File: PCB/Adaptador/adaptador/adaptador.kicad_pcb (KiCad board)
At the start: 2 copper layers, 38.1 x 41.9 mm, 4 parts

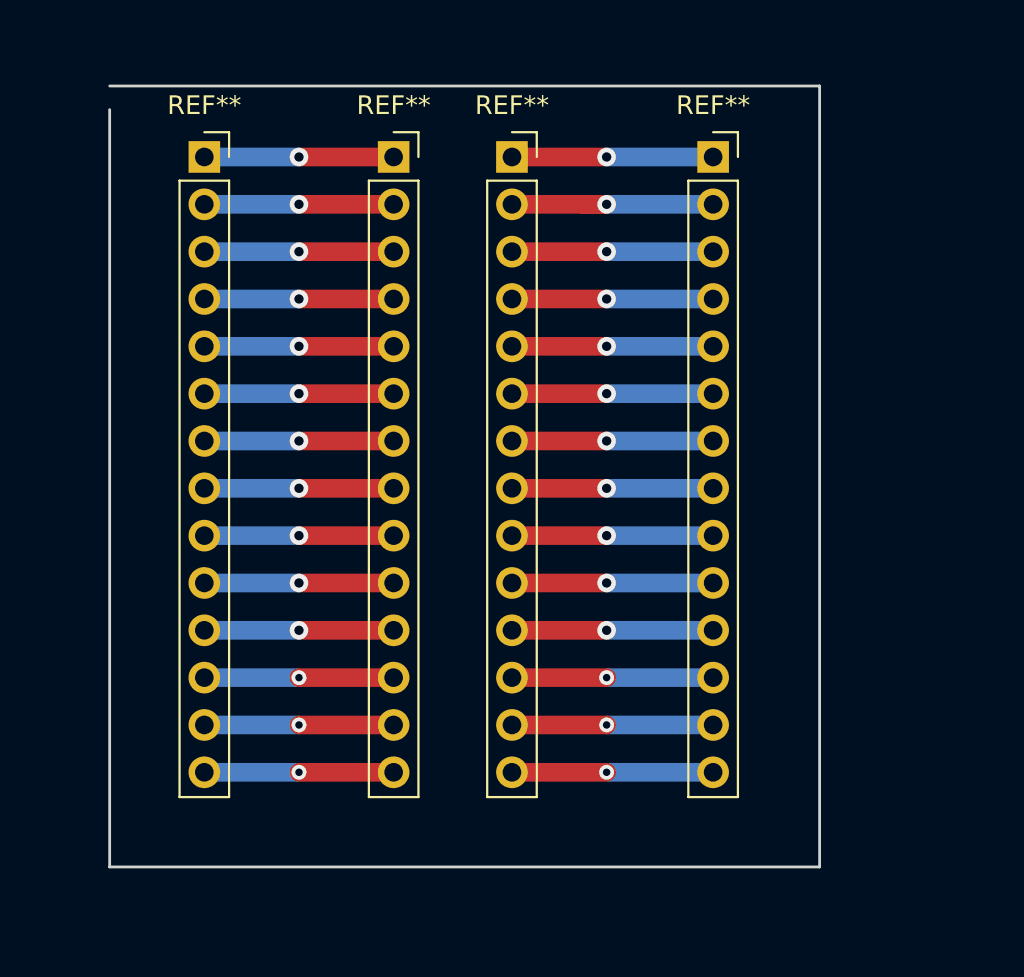
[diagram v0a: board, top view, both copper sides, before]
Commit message: Primeros prototipos de PCB para pruebas de temperatura
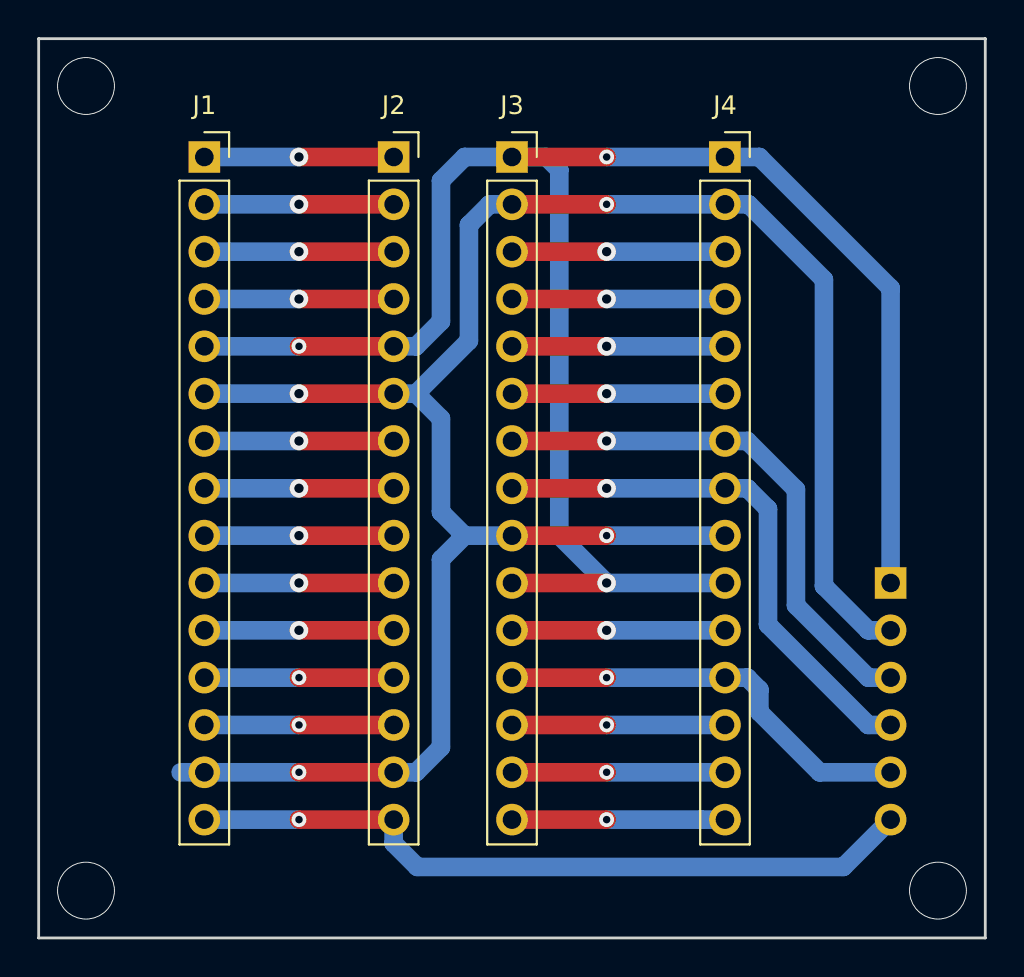
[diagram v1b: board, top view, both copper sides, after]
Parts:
- removed REF** (x4): PinSocket_1x14_P2.54mm_Vertical, Connector_PinSocket_2.54mm:PinSocket_1x14_P2.54mm_Vertical
- added J1: Conn_01x15_Female, Connector_PinSocket_2.54mm:PinSocket_1x15_P2.54mm_Vertical, F.Cu at (21.6, 21.6)
- added J2: Conn_01x15_Male, Connector_PinSocket_2.54mm:PinSocket_1x15_P2.54mm_Vertical, F.Cu at (31.8, 21.6)
- added J3: Conn_01x15_Male, Connector_PinSocket_2.54mm:PinSocket_1x15_P2.54mm_Vertical, F.Cu at (38.1, 21.6)
- added J4: Conn_01x15_Female, Connector_PinSocket_2.54mm:PinSocket_1x15_P2.54mm_Vertical, F.Cu at (49.5, 21.6)
- added J5: Conn_01x06_Male, Connector_PinSocket_2.54mm:PinSocket_1x06_P2.54mm_Horizontal, B.Cu at (58.4, 44.5)
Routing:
- net (no net): track 294.6 -> 0.00 mm, vias 28 -> 4
- net GND: track 0.00 -> 113.1 mm, vias 0 -> 4
- net VCC: track 0.00 -> 101.7 mm, vias 0 -> 3
- net /Analogo: track 0.00 -> 39.7 mm, vias 0 -> 1
- net Net-(J3-Pad8): track 0.00 -> 28.6 mm, vias 0 -> 1
- net Net-(J3-Pad7): track 0.00 -> 28.6 mm, vias 0 -> 1
- net Net-(J3-Pad12): track 0.00 -> 22.5 mm, vias 0 -> 1
- net Net-(J3-Pad15): track 0.00 -> 11.4 mm, vias 0 -> 1
- net Net-(J3-Pad14): track 0.00 -> 11.4 mm, vias 0 -> 1
- net Net-(J3-Pad13): track 0.00 -> 11.4 mm, vias 0 -> 1
- net Net-(J3-Pad6): track 0.00 -> 10.8 mm, vias 0 -> 1
- net Net-(J3-Pad5): track 0.00 -> 10.8 mm, vias 0 -> 1
- net Net-(J3-Pad4): track 0.00 -> 10.8 mm, vias 0 -> 1
- net Net-(J3-Pad3): track 0.00 -> 10.8 mm, vias 0 -> 1
- net Net-(J3-Pad11): track 0.00 -> 10.8 mm, vias 0 -> 1
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- added copper zone on B.Cu, net GND
- added copper zone on F.Cu, net VCC
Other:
- board size 38.1 x 41.9 mm -> 50.8 x 48.3 mm
